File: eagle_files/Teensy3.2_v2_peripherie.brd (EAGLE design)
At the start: 67 x 62.2 mm, 48 parts, among them IC1 L298, IC2 DS18B20, IC3 DS18B20, IC4 DS18B20

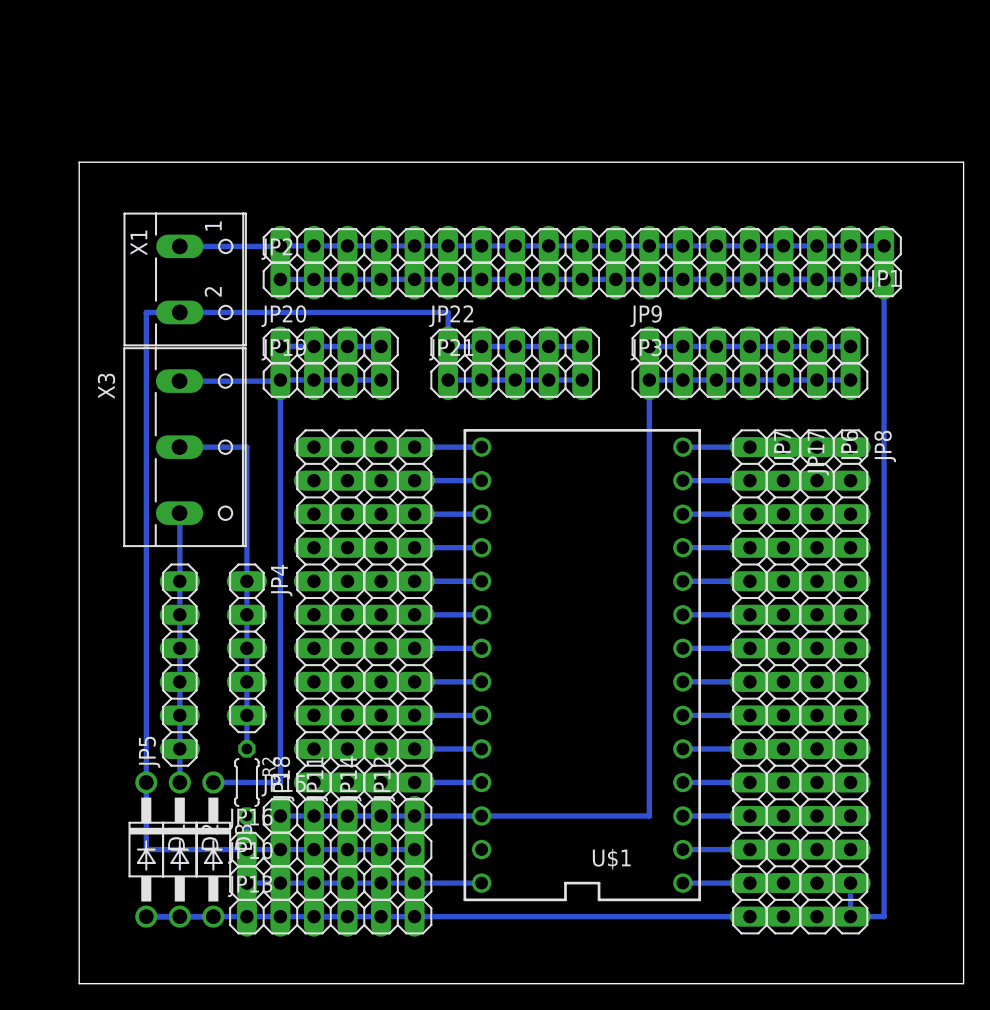
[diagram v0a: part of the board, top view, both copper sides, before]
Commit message: some edit
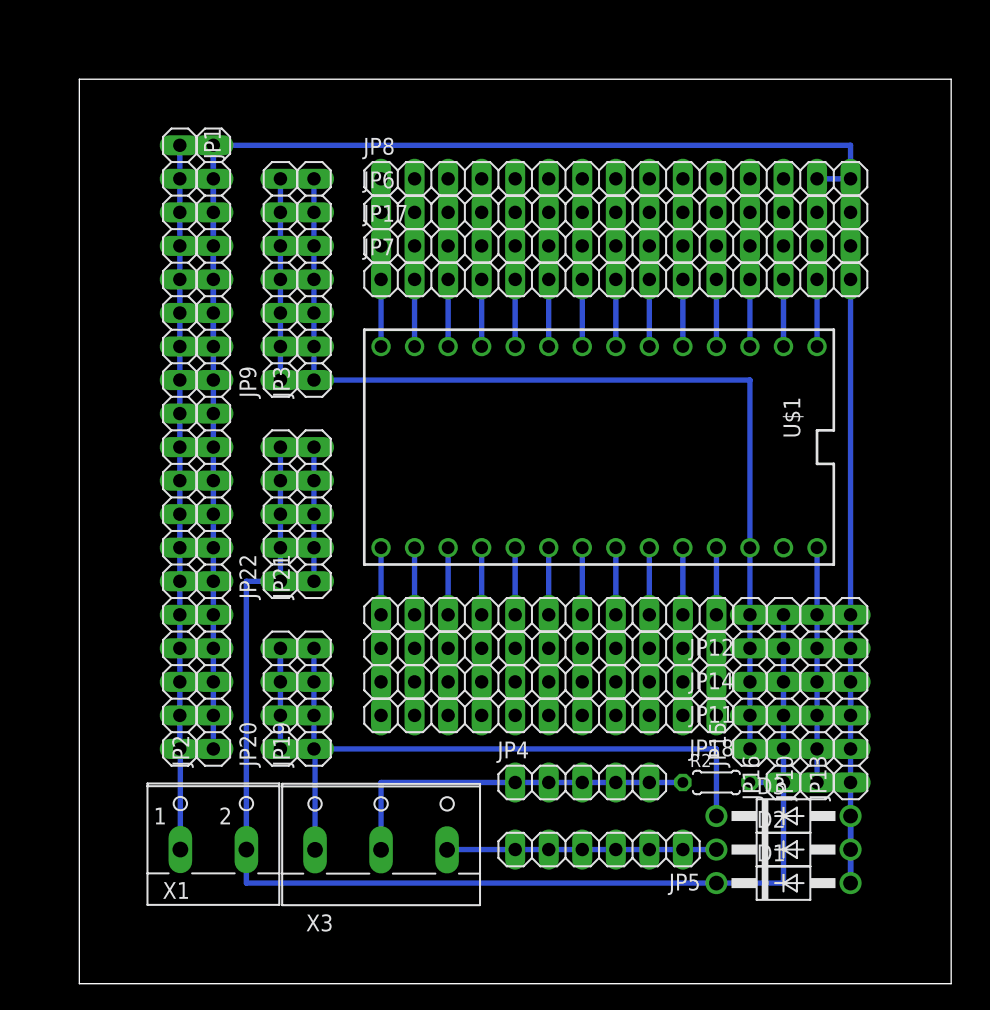
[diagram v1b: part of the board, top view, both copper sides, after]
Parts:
- moved D1 48.3 mm to (53.3, 7.62), turned to 0 degrees
- moved D2 45.7 mm to (53.3, 10.2), turned to 0 degrees
- moved D3 43.3 mm to (53.3, 12.7), turned to 0 degrees
- moved JP13 42.7 mm to (58.4, 21.6), turned to 90 degrees
- moved JP8 42.0 mm to (40.6, 61.0), turned to 0 degrees
- moved X1 41.9 mm to (10.2, 11.4), turned to 0 degrees
- moved JP10 39.4 mm to (55.9, 21.6), turned to 90 degrees
- moved JP6 38.7 mm to (40.6, 58.4), turned to 0 degrees
- moved JP16 36.1 mm to (53.3, 21.6), turned to 90 degrees
- moved JP9 35.9 mm to (15.2, 53.3), turned to 90 degrees
- moved R2 35.6 mm to (48.3, 15.2), turned to 0 degrees
- moved JP17 35.4 mm to (40.6, 55.9), turned to 0 degrees
- moved JP5 34.7 mm to (39.4, 10.2), turned to 180 degrees
- moved JP1 34.1 mm to (7.62, 40.6), turned to 270 degrees
- moved JP3 33.9 mm to (17.8, 53.3), turned to 90 degrees
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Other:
- board size 67 x 62.2 mm -> 66 x 68.5 mm
